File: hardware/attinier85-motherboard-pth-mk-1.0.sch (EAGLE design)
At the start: 9 parts, among them IC1 TINY85, U1 ATTINIER85_SHIELD

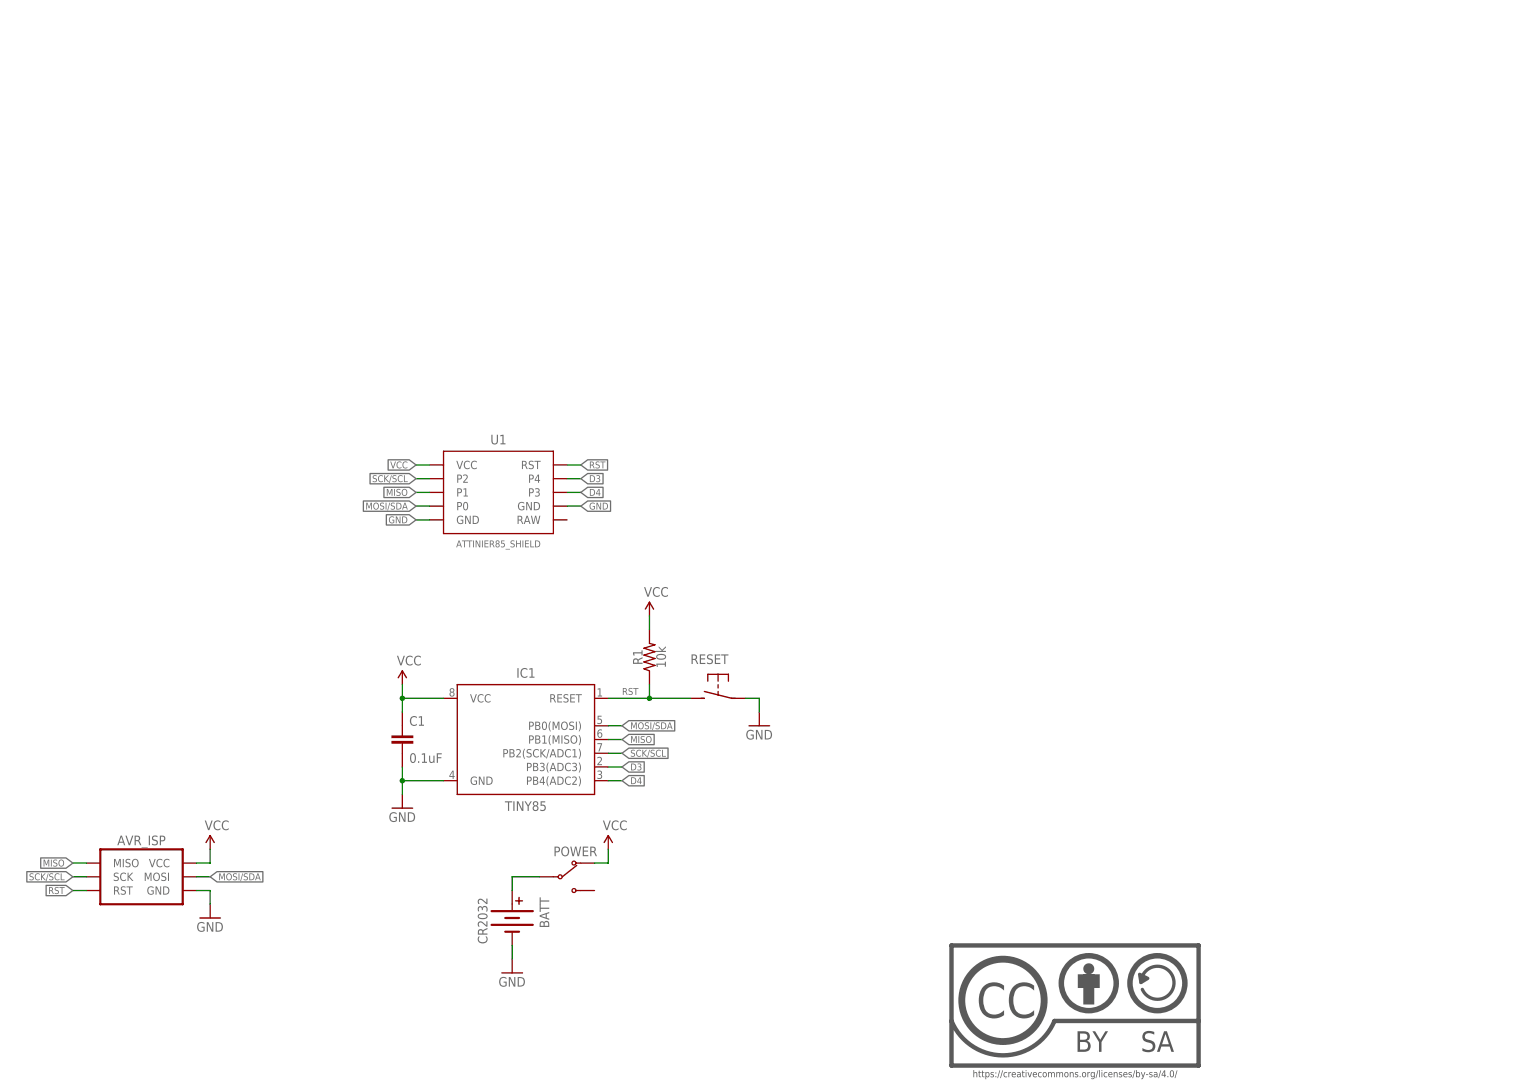
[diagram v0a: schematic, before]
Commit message: more boards
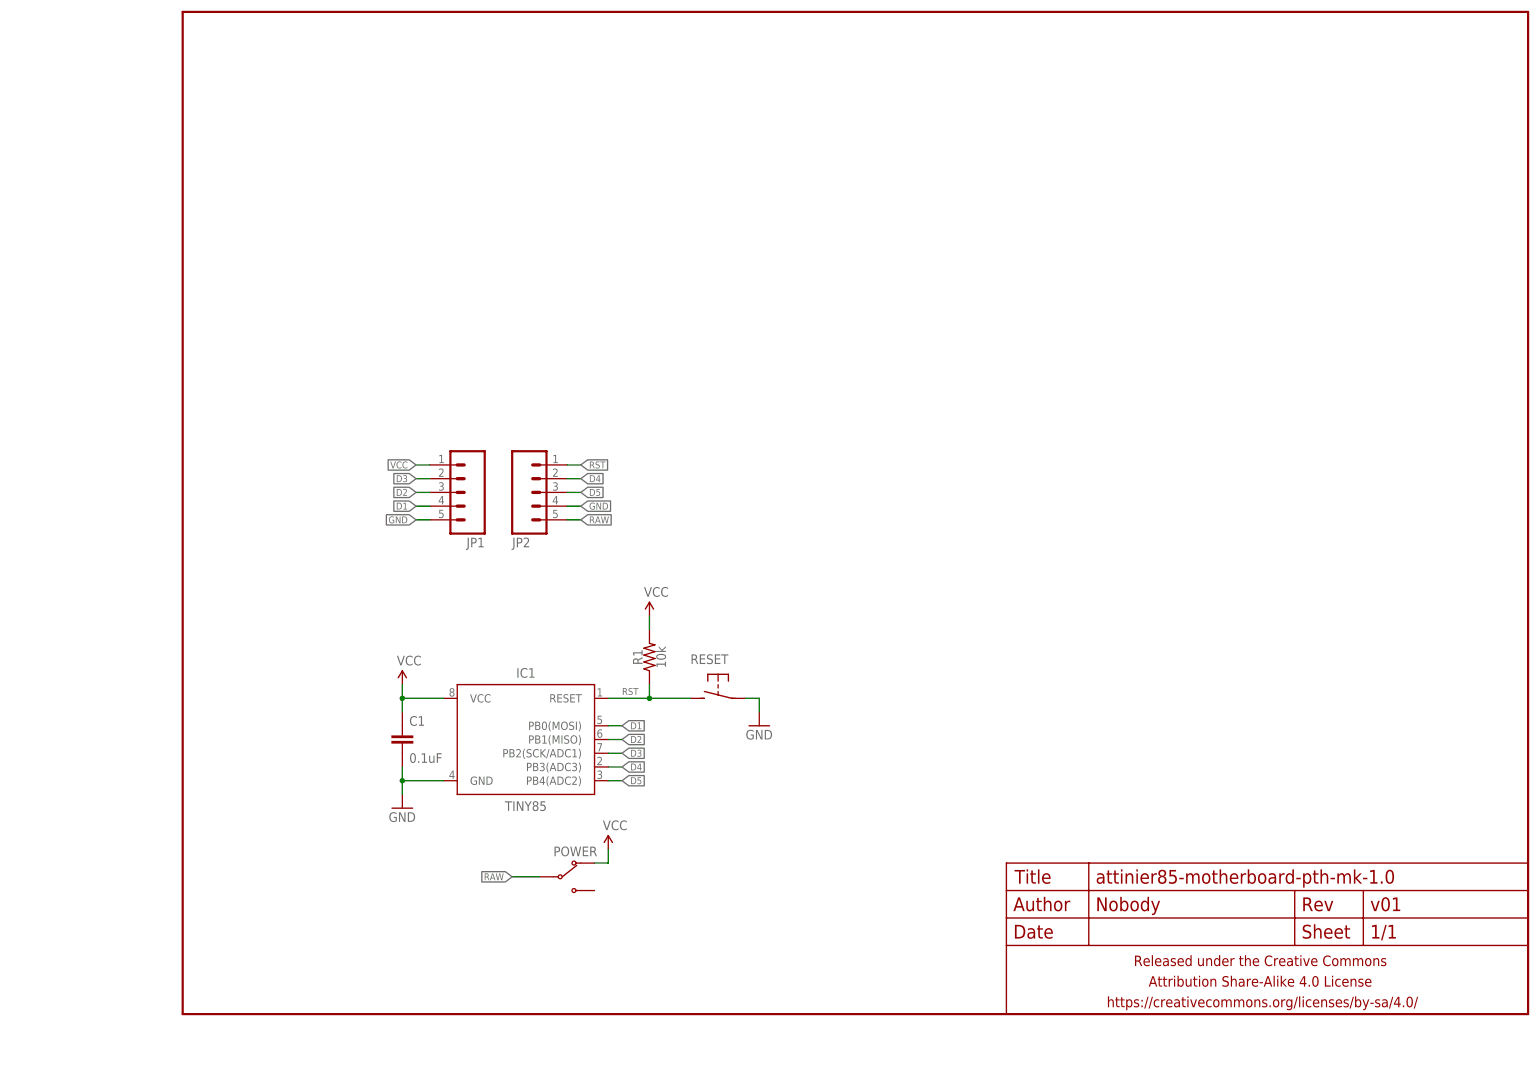
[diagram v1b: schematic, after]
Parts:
- removed AVR_ISP: AVR_SPI_PRG_6PTH, A_butts:AVR_SPI_PRG_6PTH
- removed BATT: CR2032, A_butts:BATTERY20PTH_TOPLOAD
- removed U$1: CC-BY-SA-4.0NO-URL, A_butts:CC-BY-SA-4.0NO-URL
- removed U1: ATTINIER85_SHIELD, A_butts:ATTINIER85_SHIELD
- added FRAME1: FRAME-LETTERNO_PACKAGE, a_parts:FRAME-LETTERNO_PACKAGE
- added JP1, JP2: M05PTH, a_parts:M05PTH
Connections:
- removed net MISO: AVR_ISP.MISO, IC1.PB1(MISO), U1.P1
- removed net MOSI/SDA: AVR_ISP.MOSI, IC1.PB0(MOSI), U1.P0
- removed net N$1: BATT.+, POWER.COM
- removed net SCK/SCL: AVR_ISP.SCK, IC1.PB2(SCK/ADC1), U1.P2
- new net D1: IC1.PB0(MOSI), JP1.4
- new net D2: IC1.PB1(MISO), JP1.3
- new net D5: IC1.PB4(ADC2), JP2.3
- new net RAW: JP2.5, POWER.COM
- net D3: now also IC1.PB2(SCK/ADC1), JP1.2; no longer IC1.PB3(ADC3), U1.P4
- net D4: now also IC1.PB3(ADC3), JP2.2; no longer IC1.PB4(ADC2), U1.P3
- net GND: now also JP1.5, JP2.4; no longer AVR_ISP.GND, BATT.-, U1.GND@1, U1.GND@2
- net RST: now also JP2.1; no longer AVR_ISP.RST, U1.RST
- net VCC: now also JP1.1; no longer AVR_ISP.VCC, U1.VCC
